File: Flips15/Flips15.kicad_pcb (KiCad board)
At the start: 2 copper layers, 100 x 100 mm, 59 parts, among them CN1 UFP2810, U1001 74HC238, U1002 ULN2803A, U1003 74HC238, U1004 TBD62783A, U1101 74HC238, U1102 ULN2803A, U1103 74HC238, U1104 TBD62783A, U701 74HC238, U801 74HC238, U802 ULN2803A, U803 74HC238, U804 TBD62783A, U901 74HC238, U902 ULN2803A, U903 74HC238, U904 TBD62783A

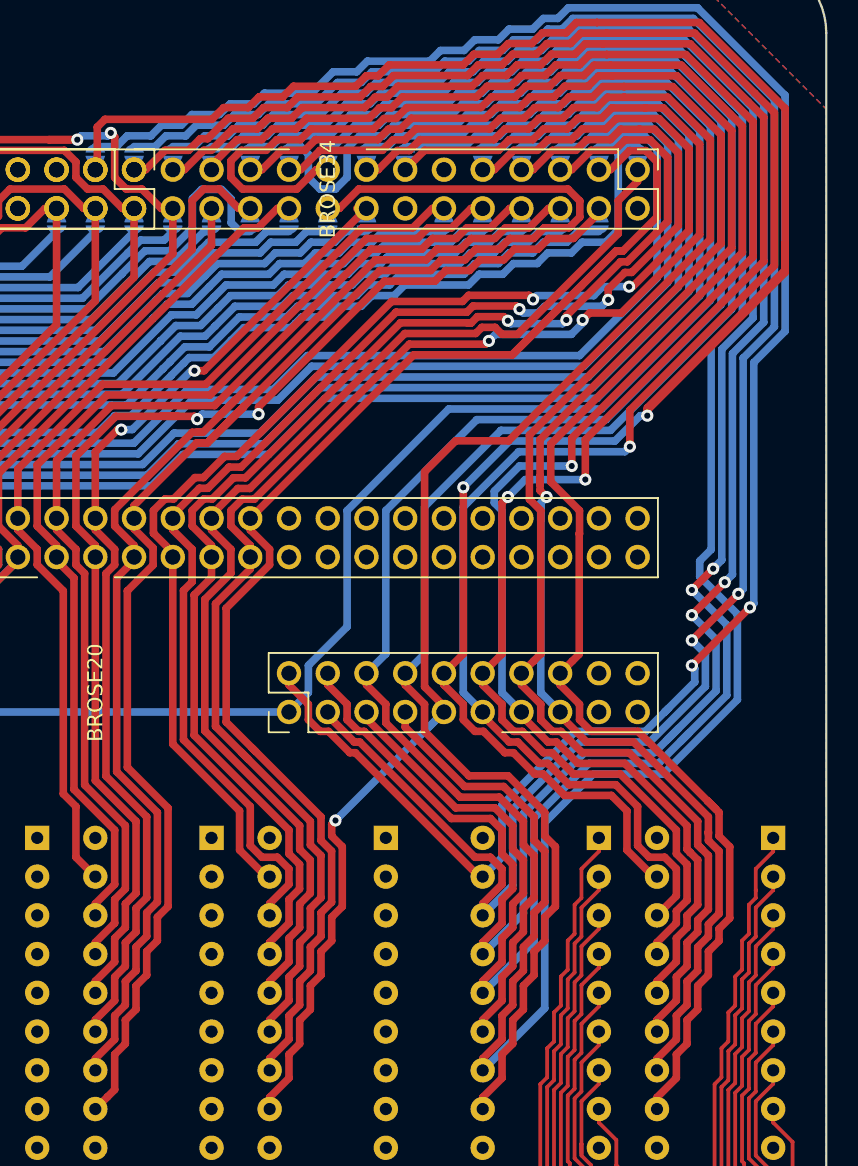
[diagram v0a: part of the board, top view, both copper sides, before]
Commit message: tracing Flips15
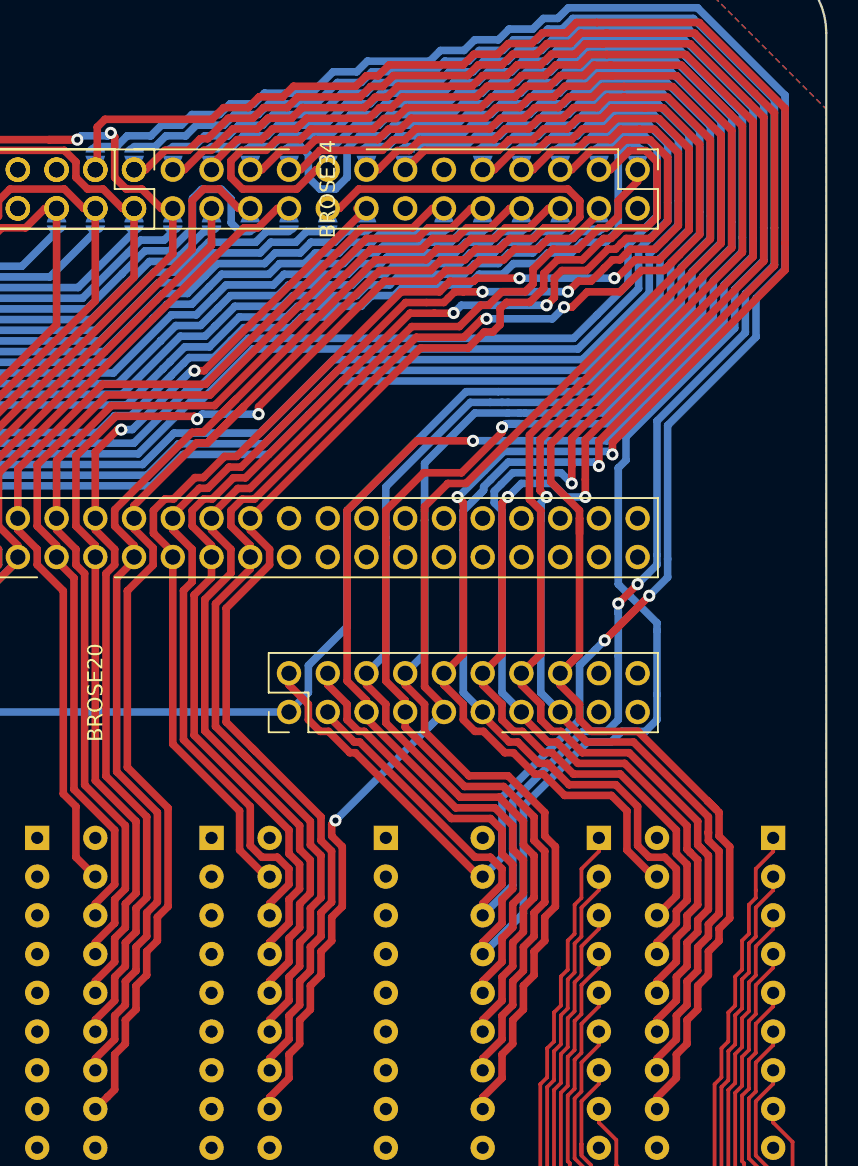
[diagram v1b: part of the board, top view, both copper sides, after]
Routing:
- net /SY27: track 147.9 -> 129.1 mm, vias 0 -> 1
- net /X22: track 140.8 -> 126.3 mm
- net /SY25: track 137.6 -> 125.3 mm, vias 2 -> 1
- net /X20: track 97.7 -> 87.7 mm
- net /X28: track 126.2 -> 129.0 mm
- net /SY23: track 131.9 -> 129.6 mm
- net /X24: track 118.5 -> 119.9 mm
- net /X19: track 106.7 -> 108.1 mm
- net /X21: track 106.7 -> 105.3 mm
- net /X25: track 115.6 -> 116.9 mm
- net /SY24: track 138.5 -> 137.5 mm, vias 2 -> 0
- net /SY19: track 130.9 -> 130.0 mm
- net /SY21: track 142.5 -> 141.6 mm
- net /SY20: track 118.0 -> 117.1 mm
- net /SY17: track 112.8 -> 111.9 mm
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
